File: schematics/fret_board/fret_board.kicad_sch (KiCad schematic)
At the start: 1 part, among them U1 Raspberry_Pi_Pico

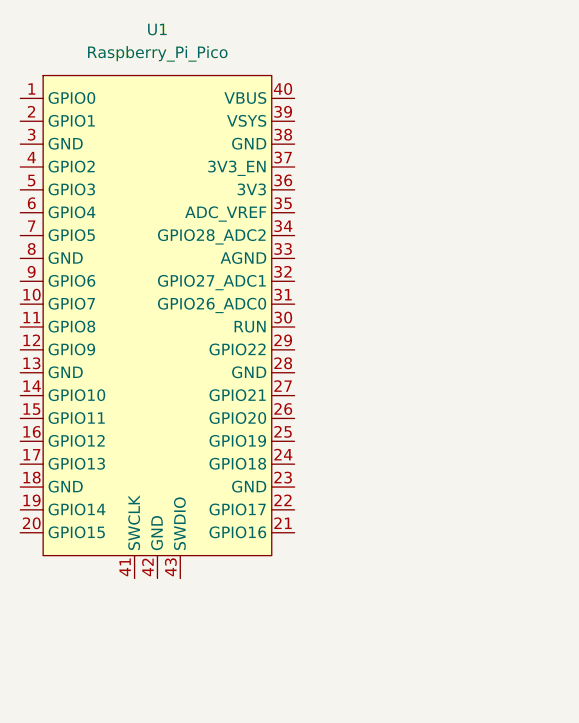
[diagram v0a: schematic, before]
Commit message: Added schematic and PCB design to fret_board
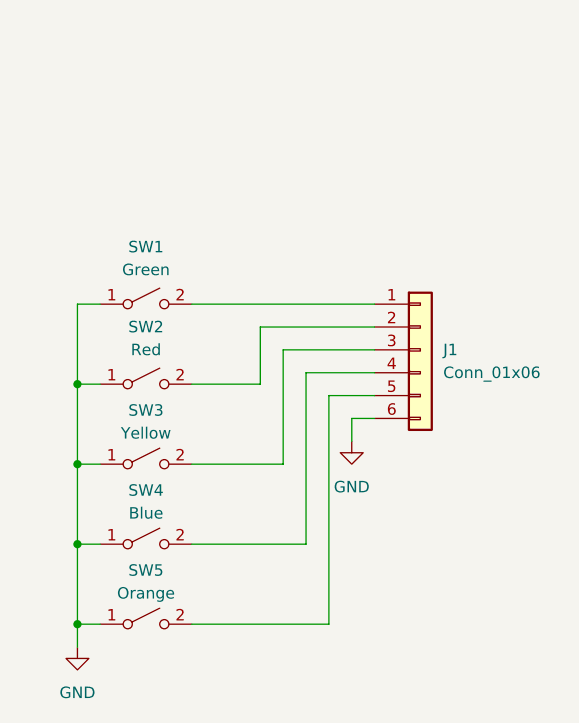
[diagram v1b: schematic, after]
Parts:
- removed U1: Raspberry_Pi_Pico, ScottoKeebs_MCU:Raspberry_Pi_Pico, symbol ScottoKeebs:MCU_Raspberry_Pi_Pico
- added J1: Conn_01x06, Connector_PinHeader_2.00mm:PinHeader_1x06_P2.00mm_Vertical, symbol Connector_Generic:Conn_01x06
- added SW1: Green, ScottoKeebs_Choc:Choc_V1, symbol Switch:SW_SPST
- added SW2: Red, ScottoKeebs_Choc:Choc_V1, symbol Switch:SW_SPST
- added SW3: Yellow, ScottoKeebs_Choc:Choc_V1, symbol Switch:SW_SPST
- added SW4: Blue, ScottoKeebs_Choc:Choc_V1, symbol Switch:SW_SPST
- added SW5: Orange, ScottoKeebs_Choc:Choc_V1, symbol Switch:SW_SPST
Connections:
- new net: J1.1 (Pin_1), SW1.2 (B)
- new net: J1.2 (Pin_2), SW2.2 (B)
- new net: J1.3 (Pin_3), SW3.2 (B)
- new net: J1.4 (Pin_4), SW4.2 (B)
- new net: J1.5 (Pin_5), SW5.2 (B)
- new net GND: J1.6 (Pin_6), SW1.1 (A), SW2.1 (A), SW3.1 (A), SW4.1 (A), SW5.1 (A)
